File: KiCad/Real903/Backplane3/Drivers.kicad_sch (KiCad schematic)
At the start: 5 parts

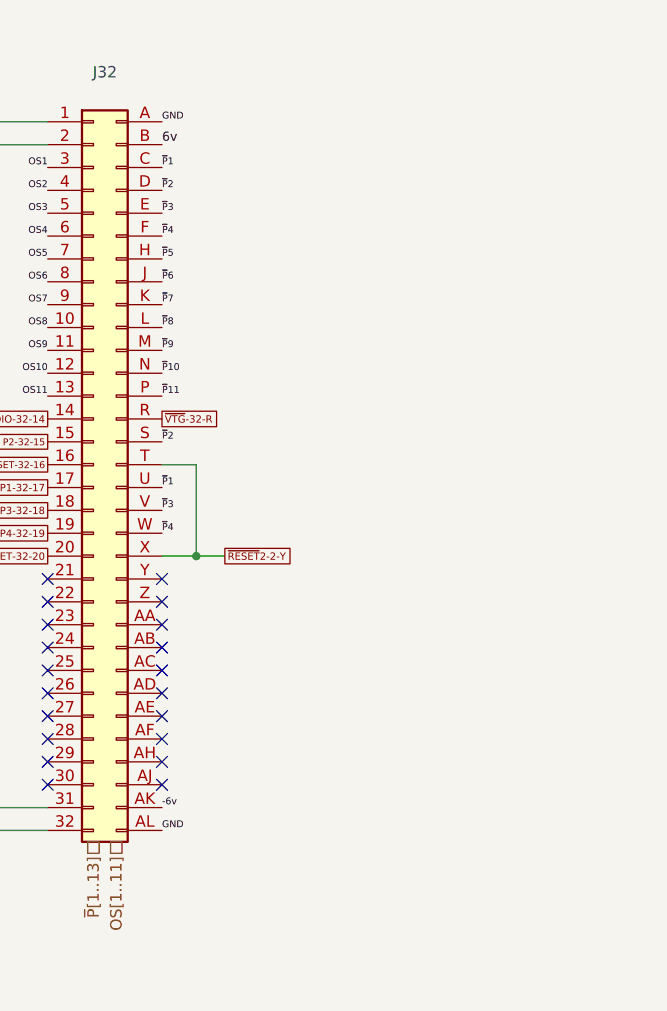
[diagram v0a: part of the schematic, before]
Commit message: Update to design
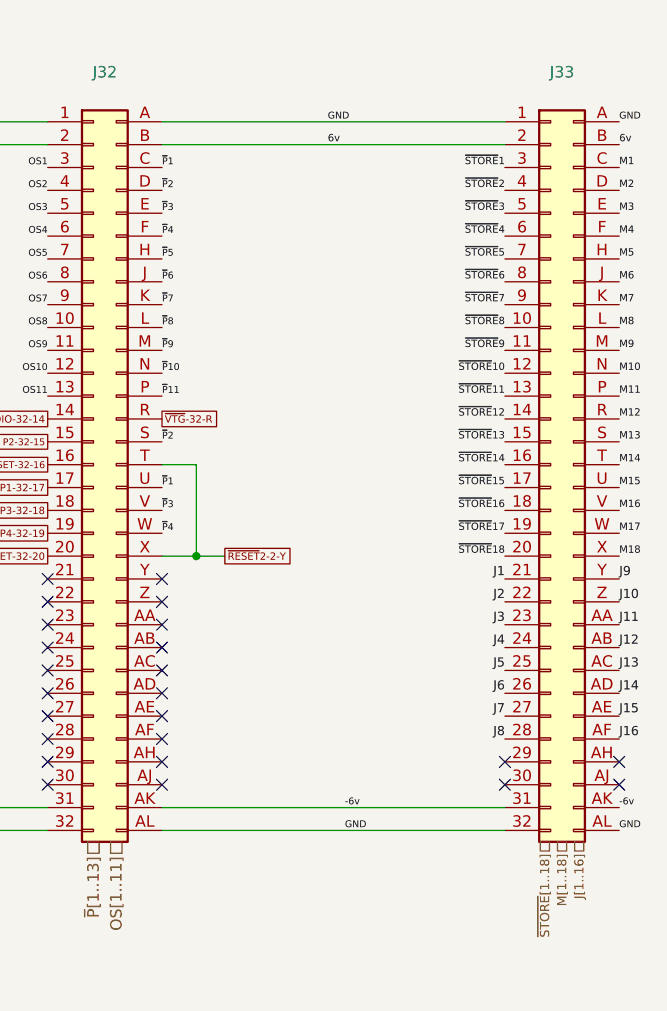
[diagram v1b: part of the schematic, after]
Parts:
- added J33: ~, ELLIOTT:DIN41612_B_2x32_Vertical, symbol LSA:Conn_02x32
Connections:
- net -6v: now also J33.31 (Pin_31), J33.AK (Pin_AK)
- net 6v: now also J33.2 (Pin_2), J33.B (Pin_B)
- net GND: now also J33.1 (Pin_1), J33.32 (Pin_32), J33.A (Pin_A), J33.AL (Pin_AL)
- new net J1: J33.21 (Pin_21)
- new net J10: J33.Z (Pin_Z)
- new net J11: J33.AA (Pin_AA)
- new net J12: J33.AB (Pin_AB)
- new net J13: J33.AC (Pin_AC)
- new net J14: J33.AD (Pin_AD)
- new net J15: J33.AE (Pin_AE)
- new net J16: J33.AF (Pin_AF)
- new net J2: J33.22 (Pin_22)
- new net J3: J33.23 (Pin_23)
- new net J4: J33.24 (Pin_24)
- new net J5: J33.25 (Pin_25)
- new net J6: J33.26 (Pin_26)
- new net J7: J33.27 (Pin_27)
- new net J8: J33.28 (Pin_28)
- new net J9: J33.Y (Pin_Y)
- new net M1: J33.C (Pin_C)
- new net M10: J33.N (Pin_N)
- new net M11: J33.P (Pin_P)
- new net M12: J33.R (Pin_R)
- new net M13: J33.S (Pin_S)
- new net M14: J33.T (Pin_T)
- new net M15: J33.U (Pin_U)
- new net M16: J33.V (Pin_V)
- new net M17: J33.W (Pin_W)
- new net M18: J33.X (Pin_X)
- new net M2: J33.D (Pin_D)
- new net M3: J33.E (Pin_E)
- new net M4: J33.F (Pin_F)
- new net M5: J33.H (Pin_H)
- new net M6: J33.J (Pin_J)
- new net M7: J33.K (Pin_K)
- new net M8: J33.L (Pin_L)
- new net M9: J33.M (Pin_M)
- new net ~{STORE}1: J33.3 (Pin_3)
- new net ~{STORE}10: J33.12 (Pin_12)
- new net ~{STORE}11: J33.13 (Pin_13)
- new net ~{STORE}12: J33.14 (Pin_14)
- new net ~{STORE}13: J33.15 (Pin_15)
- new net ~{STORE}14: J33.16 (Pin_16)
- new net ~{STORE}15: J33.17 (Pin_17)
- new net ~{STORE}16: J33.18 (Pin_18)
- new net ~{STORE}17: J33.19 (Pin_19)
- new net ~{STORE}18: J33.20 (Pin_20)
- new net ~{STORE}2: J33.4 (Pin_4)
- new net ~{STORE}3: J33.5 (Pin_5)
- new net ~{STORE}4: J33.6 (Pin_6)
- new net ~{STORE}5: J33.7 (Pin_7)
- new net ~{STORE}6: J33.8 (Pin_8)
- new net ~{STORE}7: J33.9 (Pin_9)
- new net ~{STORE}8: J33.10 (Pin_10)
- new net ~{STORE}9: J33.11 (Pin_11)
- no-connect marks 79 -> 83
